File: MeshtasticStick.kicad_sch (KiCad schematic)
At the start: 36 parts, among them J1 Conn_02x05_Odd_Even, J2 Conn_01x04, J4 Conn_01x04, J5 TYPE-C-31-M-12, U1 MDBT50Q-P1MV2, U2 E22-900M30S, U3 MP2338GTL, U4 AP2112K-3.3, Y1 Crystal

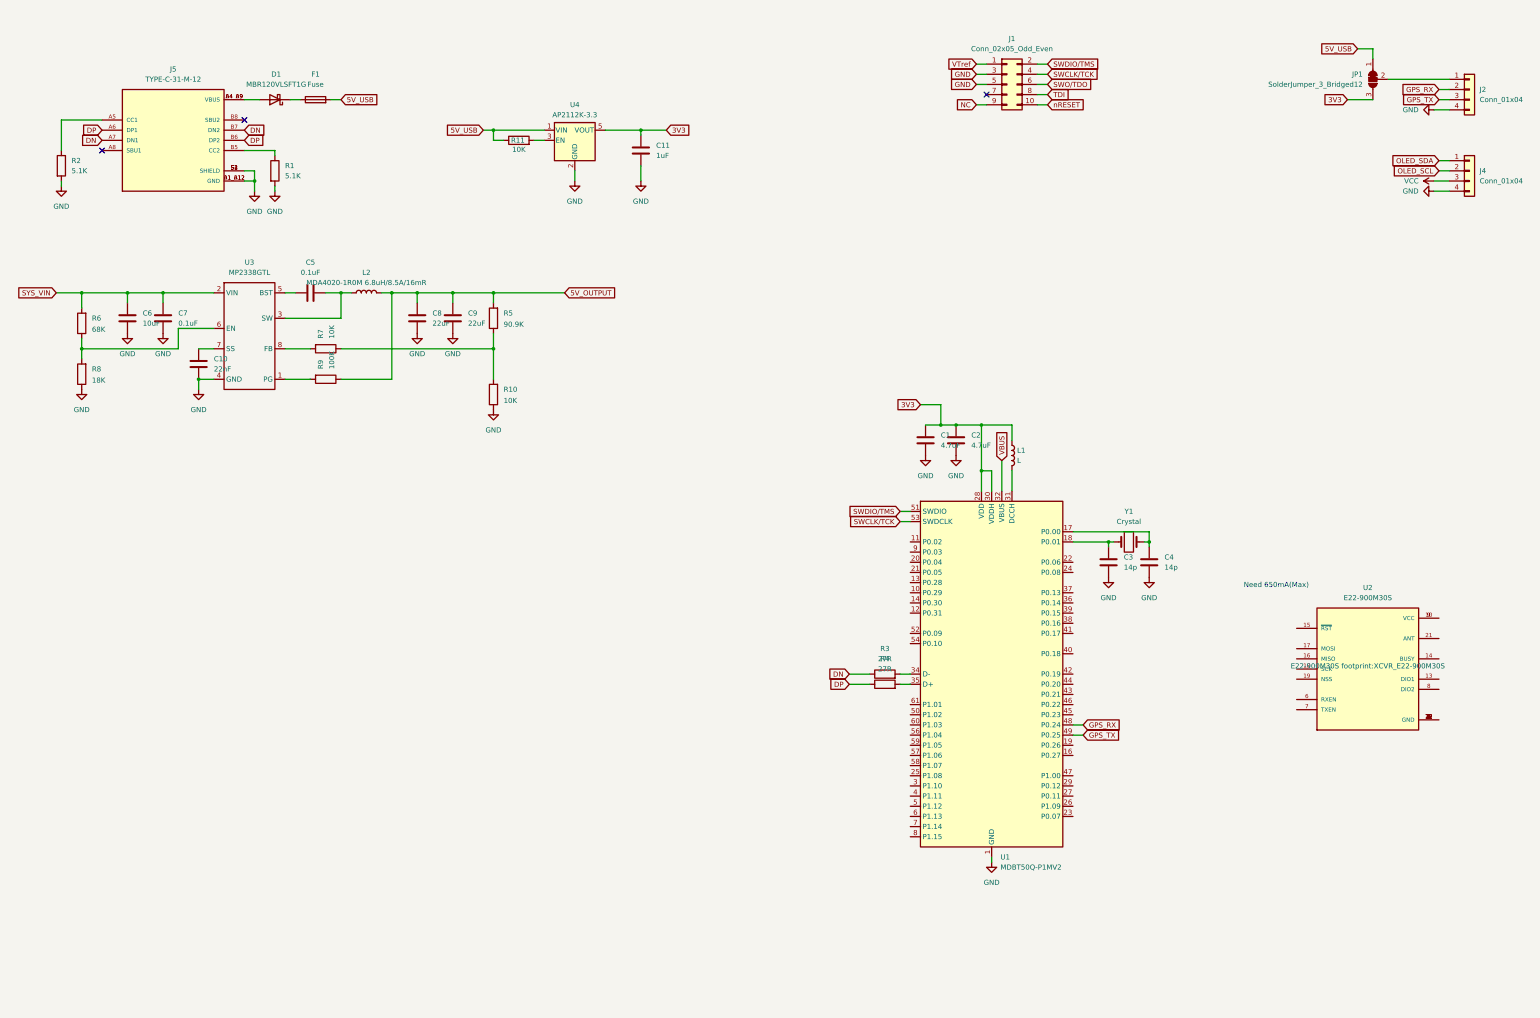
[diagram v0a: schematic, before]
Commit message: ver1
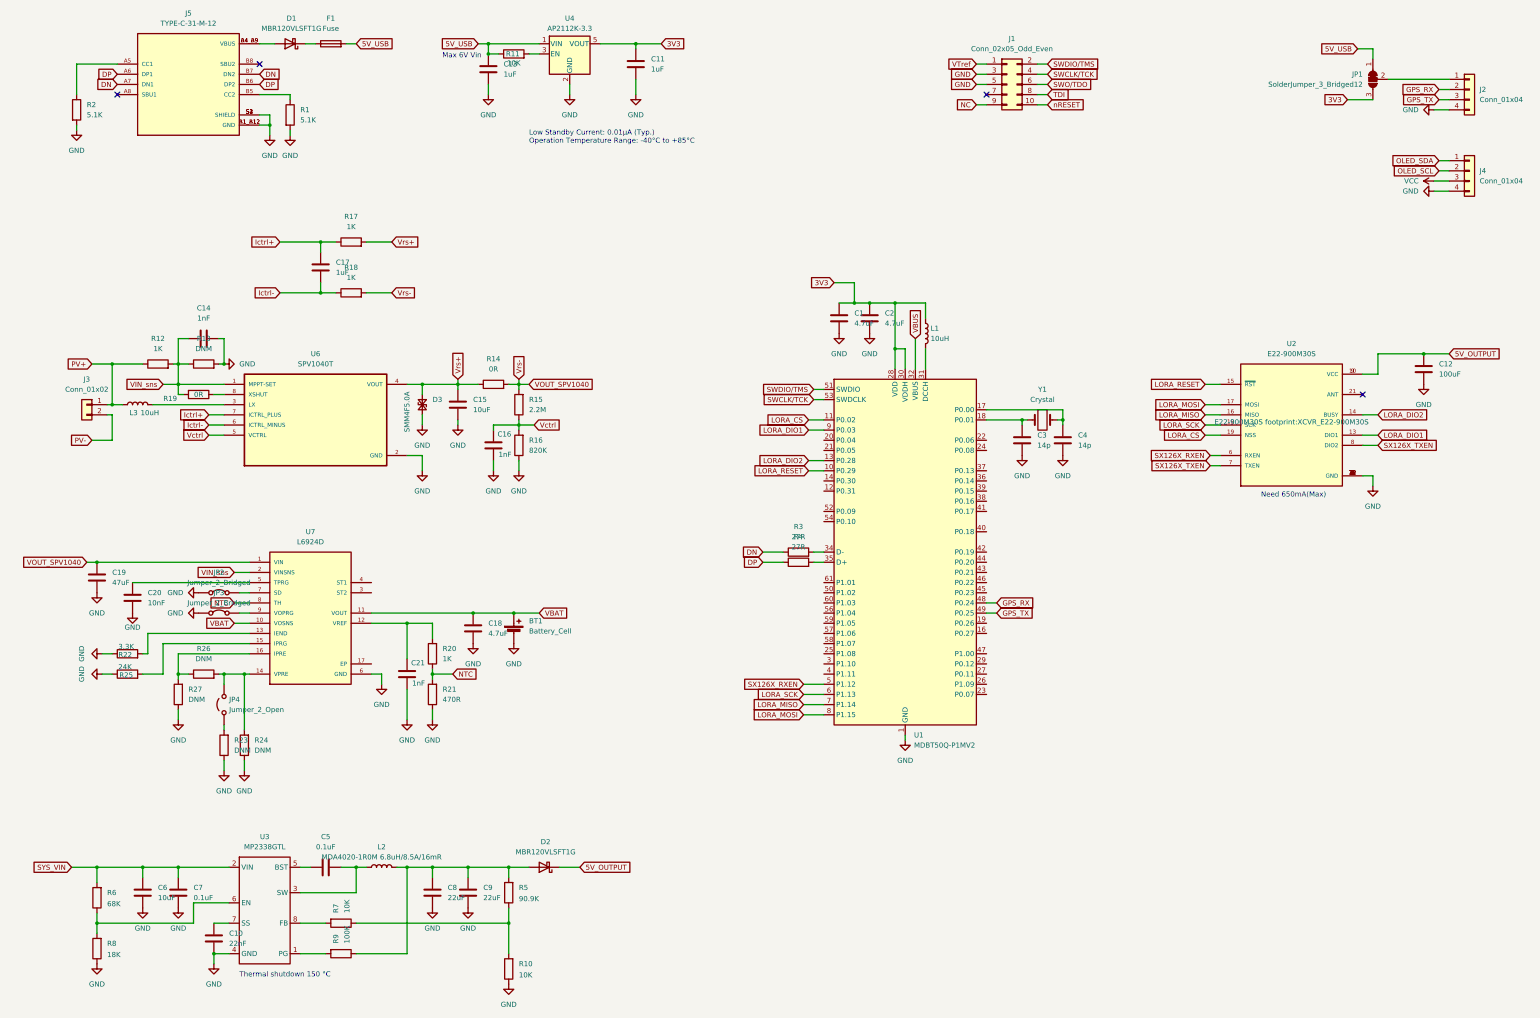
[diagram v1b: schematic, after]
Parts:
- added BT1: Battery_Cell, Connector_PinHeader_2.54mm:PinHeader_1x02_P2.54mm_Vertical, symbol Device:Battery_Cell
- added C12: 100uF, Capacitor_SMD:CP_Elec_6.3x7.7, symbol Device:C
- added C13: 1uF, Capacitor_SMD:C_0603_1608Metric, symbol Device:C
- added C14, C16: 1nF, Capacitor_SMD:C_0201_0603Metric, symbol Device:C
- added C15: 10uF, Capacitor_SMD:C_0201_0603Metric, symbol Device:C
- added C17: 1uF, Capacitor_SMD:C_0201_0603Metric, symbol Device:C
- added C18: 4.7uF, Capacitor_SMD:C_0603_1608Metric, symbol Device:C
- added C19: 47uF, Capacitor_SMD:CP_Elec_6.3x7.7, symbol Device:C
- added C20: 10nF, Capacitor_SMD:C_0603_1608Metric, symbol Device:C
- added C21: 1nF, Capacitor_SMD:C_0603_1608Metric, symbol Device:C
- added D2: MBR120VLSFT1G, Diode_SMD:D_SOD-123F, symbol Device:D_Schottky
- added D3: SMM4F5.0A, Diode_SMD:D_SMP_DO-220AA, symbol Device:D_TVS_Small
- added J3: Conn_01x02, Connector_PinHeader_2.54mm:PinHeader_1x02_P2.54mm_Vertical, symbol Connector_Generic:Conn_01x02
- added JP2, JP3: Jumper_2_Bridged, Jumper:SolderJumper-2_P1.3mm_Bridged2Bar_RoundedPad1.0x1.5mm, symbol Jumper:Jumper_2_Bridged
- added JP4: Jumper_2_Open, Jumper:SolderJumper-2_P1.3mm_Open_RoundedPad1.0x1.5mm, symbol Jumper:Jumper_2_Open
- added L3: 10uH, Fuse:Fuse_1210_3225Metric, symbol Device:L
- added R12, R17, R18, R20: 1K, Capacitor_SMD:C_0603_1608Metric, symbol Device:R
- added R13, R23, R24, R26, R27: DNM, Capacitor_SMD:C_0603_1608Metric, symbol Device:R
- added R14, R19: 0R, Capacitor_SMD:C_0603_1608Metric, symbol Device:R
- added R15: 2.2M, Capacitor_SMD:C_0603_1608Metric, symbol Device:R
- added R16: 820K, Capacitor_SMD:C_0603_1608Metric, symbol Device:R
- added R21: 470R, Capacitor_SMD:C_0603_1608Metric, symbol Device:R
- added R22: 3.3K, Capacitor_SMD:C_0603_1608Metric, symbol Device:R
- added R25: 24K, Capacitor_SMD:C_0603_1608Metric, symbol Device:R
- added U6: SPV1040T, STMicroelectronics SPV1040T:SOP65P640X120-8N, symbol SPV1040T:SPV1040T
- added U7: L6924D, L6924D footprint:QFN50P300X300X100-17N, symbol L6924D:L6924D
- C3, C4: footprint (none) -> Capacitor_SMD:C_0603_1608Metric
- D1: footprint (none) -> Diode_SMD:D_SOD-123F
- F1: footprint (none) -> Fuse:Fuse_1210_3225Metric
- J1: footprint (none) -> Connector_PinHeader_1.27mm:PinHeader_2x05_P1.27mm_Vertical
- J2, J4: footprint (none) -> Connector_PinHeader_2.54mm:PinHeader_1x04_P2.54mm_Vertical
- J5: footprint TYPE-C-31-M-12:HRO_TYPE-C-31-M-12 -> TYPE-C-31-M-12 footprint:HRO_TYPE-C-31-M-12
- JP1: footprint (none) -> Jumper:SolderJumper-3_P1.3mm_Open_RoundedPad1.0x1.5mm
- L1: value L -> 10uH; footprint (none) -> Inductor_SMD:L_1210_3225Metric
- R10, R5, R6, R7, R8, R9: footprint Resistor_SMD:R_0603_1608Metric -> Capacitor_SMD:C_0603_1608Metric
- Y1: footprint (none) -> Crystal:Crystal_SMD_2012-2Pin_2.0x1.2mm
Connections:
- net 5V_OUTPUT: now also U2.10 (VCC), U2.9 (VCC), C12.1, D2.1 (K); no longer C8.1, C9.1, L2.2, R5.2, R9.1
- net 5V_USB: now also C13.1
- net GND: now also U2.1 (GND), U2.11 (GND), U2.12 (GND), U2.2 (GND), U2.20 (GND), U2.22 (GND), U2.3 (GND), U2.4 (GND), U2.5 (GND), BT1.2 (-), C12.2, C13.2, C14.2, C15.2, C16.2, C18.2, C19.2, C20.2, C21.2, D3.2 (A2), JP2.1 (A), JP3.1 (A), R13.2, R16.1, R21.1, R22.1, R23.1, R24.1, R25.1, R27.1, U6.2 (GND), U7.6 (GND)
- net LORA_DIO1: now reaches U2.13 (DIO1)
- net LORA_DIO1: now also U1.9 (P0.03)
- net LORA_DIO2: now reaches U2.14 (BUSY)
- net LORA_DIO2: now also U1.13 (P0.28)
- net LORA_RESET: now reaches U2.15 (~{RST})
- net LORA_RESET: now also U1.10 (P0.29)
- net LORA_MISO: now reaches U2.16 (MISO)
- net LORA_MISO: now also U1.7 (P1.14)
- net LORA_MOSI: now reaches U2.17 (MOSI)
- net LORA_MOSI: now also U1.8 (P1.15)
- net LORA_SCK: now reaches U2.18 (SCK)
- net LORA_SCK: now also U1.6 (P1.13)
- net LORA_CS: now reaches U2.19 (NSS)
- net LORA_CS: now also U1.11 (P0.02)
- net SX126X_RXEN: now reaches U2.6 (RXEN)
- net SX126X_RXEN: now also U1.5 (P1.12)
- net SX126X_TXEN: now reaches U2.7 (TXEN)
- net SX126X_TXEN: now also U2.8 (DIO2)
- new net: JP4.1 (A), R23.2
- new net: JP4.2 (B), R24.2, R26.2, U7.14 (VPRE)
- new net: C21.1, R20.2, U7.12 (VREF)
- new net: R22.2, U7.13 (IEND)
- new net: R25.2, U7.15 (IPRG)
- new net: R26.1, R27.2, U7.16 (IPRE)
- new net: C20.1, U7.5 (TPRG)
- new net: JP2.2 (B), U7.7 (SD)
- new net: JP3.2 (B), U7.9 (VOPRG)
- new net: C8.1, C9.1, D2.2 (A), L2.2, R5.2, R9.1
- new net: L3.2, U6.3 (LX)
- new net: R19.1, U6.8 (XSHUT)
- new net Ictrl+: C17.2, R17.1, U6.7 (ICTRL_PLUS)
- new net Ictrl-: C17.1, R18.1, U6.6 (ICTRL_MINUS)
- new net NTC: R20.1, R21.2, U7.8 (TH)
- new net PV+: J3.1 (Pin_1), L3.1, R12.1
- new net PV-: J3.2 (Pin_2)
- new net VBAT: BT1.1 (+), C18.1, U7.10 (VOSNS), U7.11 (VOUT)
- new net VIN_sns: C14.1, R12.2, R13.1, R19.2, U6.1 (MPPT-SET), U7.2 (VINSNS)
- new net VOUT_SPV1040: C19.1, R14.2, R15.2, R18.2, U7.1 (VIN)
- new net Vctrl: C16.1, R15.1, R16.2, U6.5 (VCTRL)
- new net Vrs+: C15.1, D3.1 (A1), R14.1, R17.2, U6.4 (VOUT)
- no-connect marks 3 -> 4
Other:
- note added: "Low Standby Current: 0.01µA (Typ.) Operation Temperature Range: -40°C to +85°C"
- note added: "Max 6V Vin"
- note added: "Thermal shutdown 150 °C"
- moved on the sheet: C1, C10, C11, C2, C3, C4, C5, C6, C7, C8, C9, D1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
